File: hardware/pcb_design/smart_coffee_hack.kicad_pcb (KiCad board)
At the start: 2 copper layers, 54.9 x 79 mm, 17 parts, among them P1 CONN_COFFEE_MACHINE_02X04, Q1 BC547, Q2 BC547, Q3 BC547, Q4 BC547, U1 NodeMCU_Amica_R2

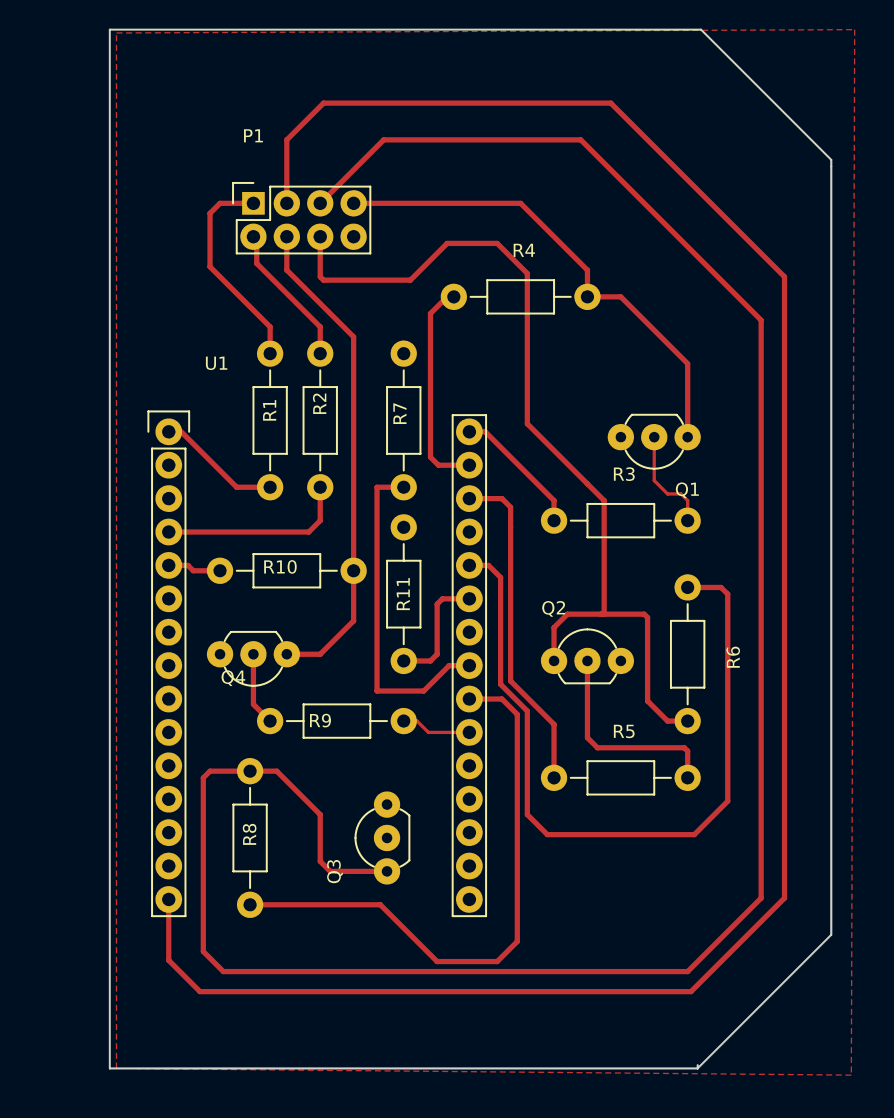
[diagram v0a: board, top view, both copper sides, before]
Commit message: PCB modification
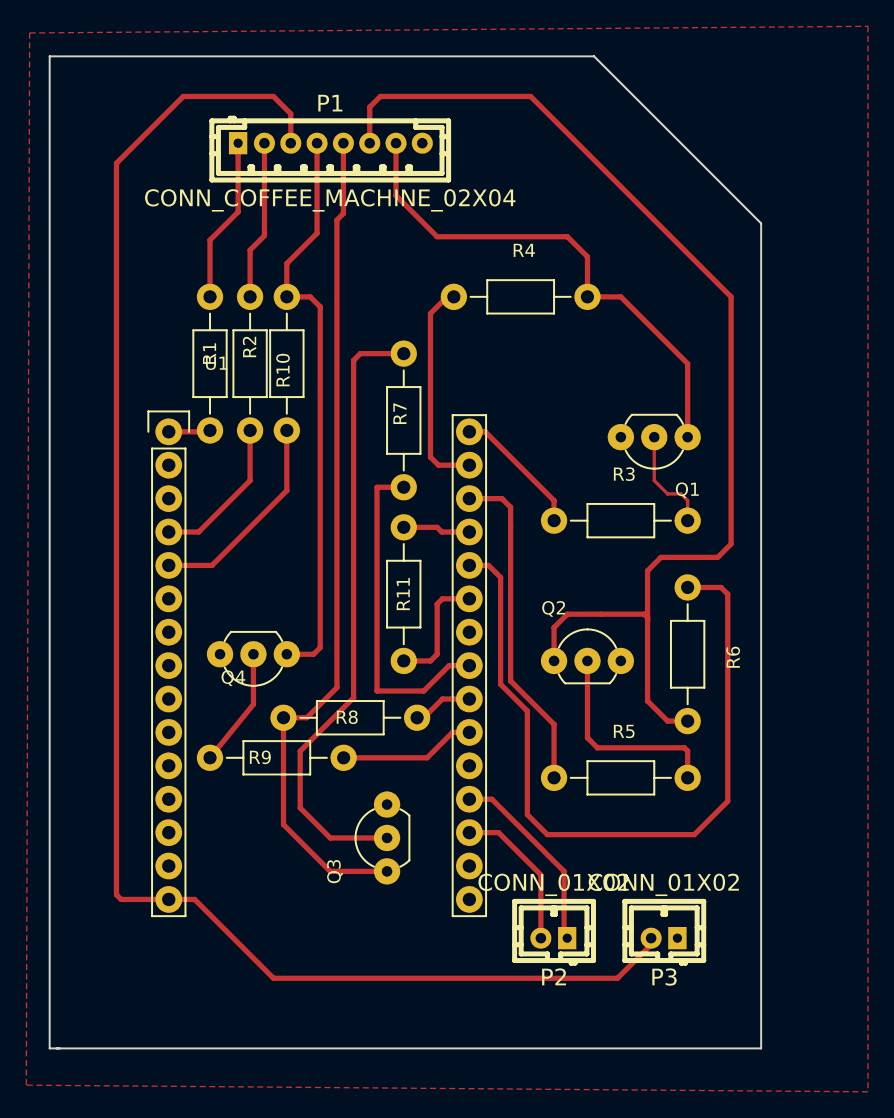
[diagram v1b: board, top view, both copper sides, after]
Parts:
- added P2: CONN_01X02, w_conn_jst-ph:b2b-ph-kl, F.Cu at (177.8, 143.5)
- added P3: CONN_01X02, w_conn_jst-ph:b2b-ph-kl, F.Cu at (186.2, 143.5)
- P1: footprint Socket_Strips:Socket_Strip_Straight_2x04 -> w_conn_jst-ph:b8b-ph-kl
- moved R8 19.1 mm to (167.4, 126.7), turned to 180 degrees
- moved R10 11.8 mm to (157.5, 104.9), turned to 90 degrees
- moved P1 7.42 mm to (160.8, 83.1)
- moved R2 6.86 mm to (154.7, 104.9)
- moved R1 6.29 mm to (151.6, 104.9)
- moved R9 5.36 mm to (161.8, 129.8)
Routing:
- net Net-(P1-Pad5): track 163.1 -> 64.1 mm
- net Net-(Q3-Pad2): track 0.00 -> 47.3 mm
- net Net-(R8-Pad1): track 44.1 -> 4.56 mm
- net +5V: track 151.9 -> 118.6 mm
- net Net-(P1-Pad6): track 69.8 -> 86.9 mm
- net Net-(P2-Pad1): track 0.00 -> 14.7 mm
- net Net-(R10-Pad1): track 4.64 -> 16.5 mm
- net Net-(P2-Pad2): track 0.00 -> 11.6 mm
- net Net-(P1-Pad4): track 37.4 -> 44.2 mm
- net Net-(R1-Pad1): track 9.46 -> 4.28 mm
- net Net-(R11-Pad2): track 0.00 -> 5.14 mm
- net Net-(R9-Pad1): track 5.35 -> 10.4 mm
- net Net-(P1-Pad1): track 16.2 -> 12.6 mm
- net Net-(Q4-Pad2): track 5.61 -> 9.05 mm
- net Net-(R2-Pad1): track 14.4 -> 11.8 mm
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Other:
- board size 54.9 x 79 mm -> 54.1 x 75.4 mm
- net class Default: clearance 0.2 -> 0.3
- rule trace_clearance: 0.2 -> 0.3
